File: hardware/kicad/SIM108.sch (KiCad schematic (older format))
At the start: 57 parts, among them J1 Screw_Terminal_01x09, Q1 BC547, Q10 BC337-40, Q11 BC547, Q12 BC337-40, Q13 BC547, Q14 BC337-40, Q15 BC547, Q16 BC337-40, Q2 BC337-40, Q3 BC547, Q4 BC337-40, Q5 BC547, Q6 BC337-40, Q7 BC547, Q8 BC337-40, Q9 BC547, U1 SFH617A-1, U2 SFH617A-1, U3 SFH617A-1, U4 SFH617A-1, U5 SFH617A-1, U6 SFH617A-1, U7 SFH617A-1, U8 SFH617A-1

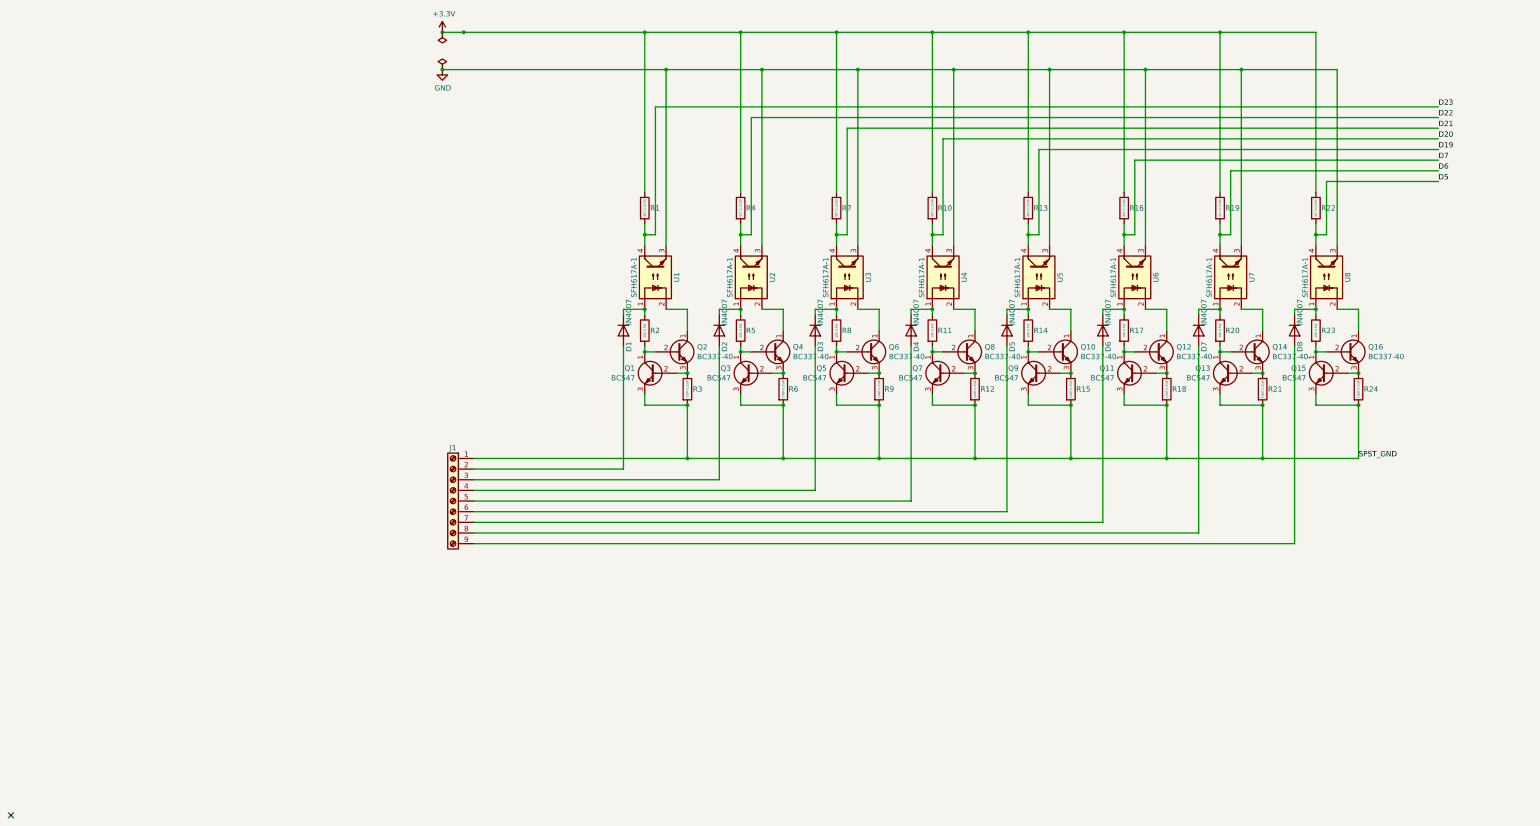
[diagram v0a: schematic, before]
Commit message: New PCB layout
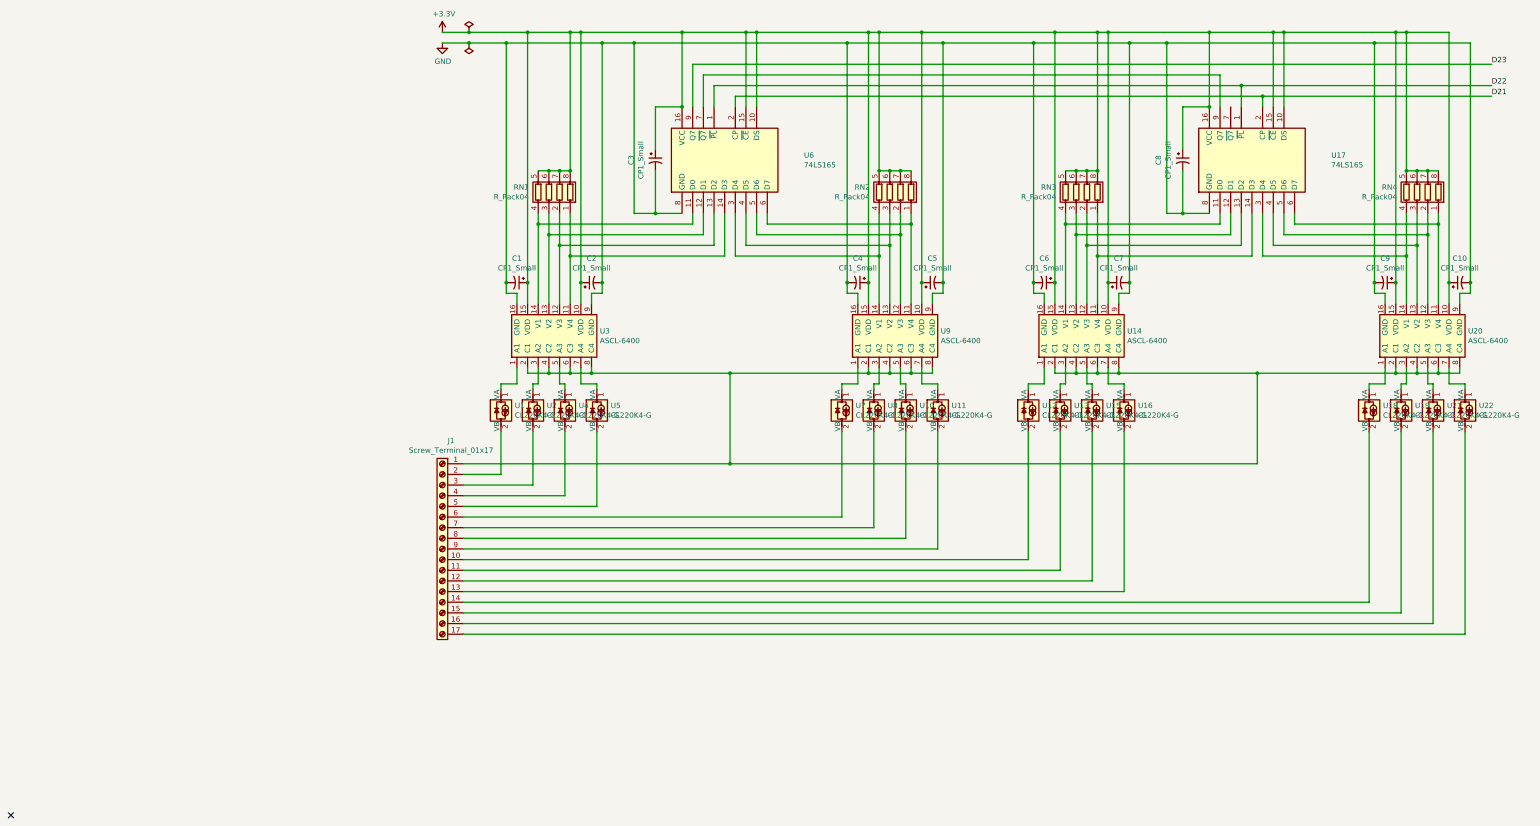
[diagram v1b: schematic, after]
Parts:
- removed D1, D2, D3, D4, D5, D6, D7, D8: IN4007, Diode_SMD:D_SOT-23_ANK, symbol Simulation_SPICE:DIODE
- removed J1: Screw_Terminal_01x09, PDJR_Connectors:CAMDEN_BOSS_CSTBV2-9_TERMINAL, symbol Connector:Screw_Terminal_01x09
- removed Q1, Q11, Q13, Q15, Q3, Q5, Q7, Q9: BC547, Package_TO_SOT_SMD:TSOT-23, symbol Transistor_BJT:BC547
- removed Q10, Q12, Q14, Q16, Q2, Q4, Q6, Q8: BC337-40, Package_TO_SOT_SMD:TSOT-23, symbol Transistor_BJT:BC337
- removed R1, R10, R13, R16, R19, R22, R4, R7: 4K7 0.125W, Resistor_SMD:R_0805_2012Metric, symbol Device:R
- removed R11, R14, R17, R2, R20, R23, R5, R8: 10K 0.5W, Resistor_SMD:R_0805_2012Metric, symbol Device:R
- removed R12, R15, R18, R21, R24, R3, R6, R9: 100R 0.25W, Resistor_SMD:R_0805_2012Metric, symbol Device:R
- removed U1, U2, U3, U4, U5, U6, U7, U8: SFH617A-1, Package_DIP:SMDIP-4_W7.62mm, symbol Isolator:SFH617A-1
- added C1, C10, C2, C3, C4, C5, C6, C7, C8, C9: CP1_Small, Capacitor_SMD:C_0504_1310Metric, symbol Device:CP1_Small
- added J1: Screw_Terminal_01x17, PDJR_Connectors:PHOENIX_SPTAF_3_5_17, symbol Connector:Screw_Terminal_01x17
- added RN1, RN2, RN3, RN4: R_Pack04, Resistor_SMD:R_Array_Convex_4x1206, symbol Device:R_Pack04
- added U1, U10, U11, U12, U13, U15, U16, U18, U19, U2, U21, U22, U4, U5, U7, U8: CL220K4-G, Package_TO_SOT_SMD:TO-252-2, symbol Driver_LED:CL220K4-G
- added U14, U20, U3, U9: ASCL-6400, Package_SO:SO-16_5.3x10.2mm_P1.27mm, symbol pdjr:ASCL-6400
- added U17, U6: 74LS165, Package_SO:SOP-16_4.4x10.4mm_P1.27mm, symbol pdjr:74LS165
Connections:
- net +3V3: now also C1.1, C10.1, C2.1, C3.1, C4.1, C5.1, C6.1, C7.1, C8.1, C9.1, RN1.5 (R4.2), RN1.6 (R3.2), RN1.7 (R2.2), RN1.8 (R1.2), RN2.5 (R4.2), RN2.6 (R3.2), RN2.7 (R2.2), RN2.8 (R1.2), RN3.5 (R4.2), RN3.6 (R3.2), RN3.7 (R2.2), RN3.8 (R1.2), RN4.5 (R4.2), RN4.6 (R3.2), RN4.7 (R2.2), RN4.8 (R1.2), U14.10 (VDD), U14.15 (VDD), U17.10 (DS), U17.15 (~CE), U17.16 (VCC), U20.10 (VDD), U20.15 (VDD), U3.10 (VDD), U3.15 (VDD), U6.10 (DS), U6.15 (~CE), U6.16 (VCC), U9.10 (VDD), U9.15 (VDD)
- net D21: now also U17.2 (CP), U6.2 (CP)
- net D22: now also U17.1 (~PL), U6.1 (~PL)
- net D23: now also U6.9 (Q7)
- net GND: now also C1.2, C10.2, C2.2, C3.2, C4.2, C5.2, C6.2, C7.2, C8.2, C9.2, U14.16 (GND), U14.9 (GND), U17.8 (GND), U20.16 (GND), U20.9 (GND), U3.16 (GND), U3.9 (GND), U6.8 (GND), U9.16 (GND), U9.9 (GND)
- new net: RN3.1 (R1.1), U14.11 (V4), U17.14 (D3)
- new net: RN3.2 (R2.1), U14.12 (V3), U17.13 (D2)
- new net: RN3.3 (R3.1), U14.13 (V2), U17.12 (D1)
- new net: RN3.4 (R4.1), U14.14 (V1), U17.11 (D0)
- new net: U2.1 (VA), U3.3 (A2)
- new net: J1.3 (Pin_3), U2.2 (VB)
- new net: U3.5 (A3), U4.1 (VA)
- new net: J1.4 (Pin_4), U4.2 (VB)
- new net: U3.7 (A4), U5.1 (VA)
- new net: J1.5 (Pin_5), U5.2 (VB)
- new net: U1.1 (VA), U3.1 (A1)
- new net: J1.2 (Pin_2), U1.2 (VB)
- new net: RN4.1 (R1.1), U17.6 (D7), U20.11 (V4)
- new net: RN4.2 (R2.1), U17.5 (D6), U20.12 (V3)
- new net: RN4.3 (R3.1), U17.4 (D5), U20.13 (V2)
- new net: RN4.4 (R4.1), U17.3 (D4), U20.14 (V1)
- new net: RN1.1 (R1.1), U3.11 (V4), U6.14 (D3)
- new net: RN1.2 (R2.1), U3.12 (V3), U6.13 (D2)
- new net: RN1.3 (R3.1), U3.13 (V2), U6.12 (D1)
- new net: RN1.4 (R4.1), U3.14 (V1), U6.11 (D0)
- new net: J1.1 (Pin_1), U14.2 (C1), U14.4 (C2), U14.6 (C3), U14.8 (C4), U20.2 (C1), U20.4 (C2), U20.6 (C3), U20.8 (C4), U3.2 (C1), U3.4 (C2), U3.6 (C3), U3.8 (C4), U9.2 (C1), U9.4 (C2), U9.6 (C3), U9.8 (C4)
- new net: U7.1 (VA), U9.1 (A1)
- new net: RN2.1 (R1.1), U6.6 (D7), U9.11 (V4)
- new net: RN2.2 (R2.1), U6.5 (D6), U9.12 (V3)
- new net: RN2.3 (R3.1), U6.4 (D5), U9.13 (V2)
- new net: RN2.4 (R4.1), U6.3 (D4), U9.14 (V1)
- new net: U8.1 (VA), U9.3 (A2)
- new net: U10.1 (VA), U9.5 (A3)
- new net: U11.1 (VA), U9.7 (A4)
- new net: U17.9 (Q7), U6.7 (~Q7)
- new net: J1.7 (Pin_7), U8.2 (VB)
- new net: J1.8 (Pin_8), U10.2 (VB)
- new net: J1.9 (Pin_9), U11.2 (VB)
- new net: J1.6 (Pin_6), U7.2 (VB)
- new net: U12.1 (VA), U14.1 (A1)
- new net: U13.1 (VA), U14.3 (A2)
- new net: U14.5 (A3), U15.1 (VA)
- new net: U14.7 (A4), U16.1 (VA)
- new net: U18.1 (VA), U20.1 (A1)
- new net: U19.1 (VA), U20.3 (A2)
- new net: U20.5 (A3), U21.1 (VA)
- new net: U20.7 (A4), U22.1 (VA)
- new net: J1.11 (Pin_11), U13.2 (VB)
- new net: J1.12 (Pin_12), U15.2 (VB)
- new net: J1.13 (Pin_13), U16.2 (VB)
- new net: J1.10 (Pin_10), U12.2 (VB)
- new net: J1.15 (Pin_15), U19.2 (VB)
- new net: J1.16 (Pin_16), U21.2 (VB)
- new net: J1.17 (Pin_17), U22.2 (VB)
- new net: J1.14 (Pin_14), U18.2 (VB)
